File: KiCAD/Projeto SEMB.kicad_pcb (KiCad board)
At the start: 2 copper layers, 153 x 122.5 mm, 90 parts, among them J1 Battery-12V, J2 ST-Link V2, M1 Motor_DC, Q1 IRLML5203, Q2 IRF740, Q3 IRF740, Q4 IRF740, Q5 IRF740, Q6 IRF740, Q7 IRF740, Q8 IRF740, Q9 IRF740, SW1 Reset, SW2 BOOT_0, SW3 SW_SPDT, SW4 User Button, U1 STM32F411CEUx, U10 XL4015, U11 LCD-016N002L, U13 INA333xxDGK, U2 2SMPP-03, U3 TLV2371P, U4 DRV8212P, U5 PCF8574A, U7 TPS7A2433DBVR, Y1 LSE

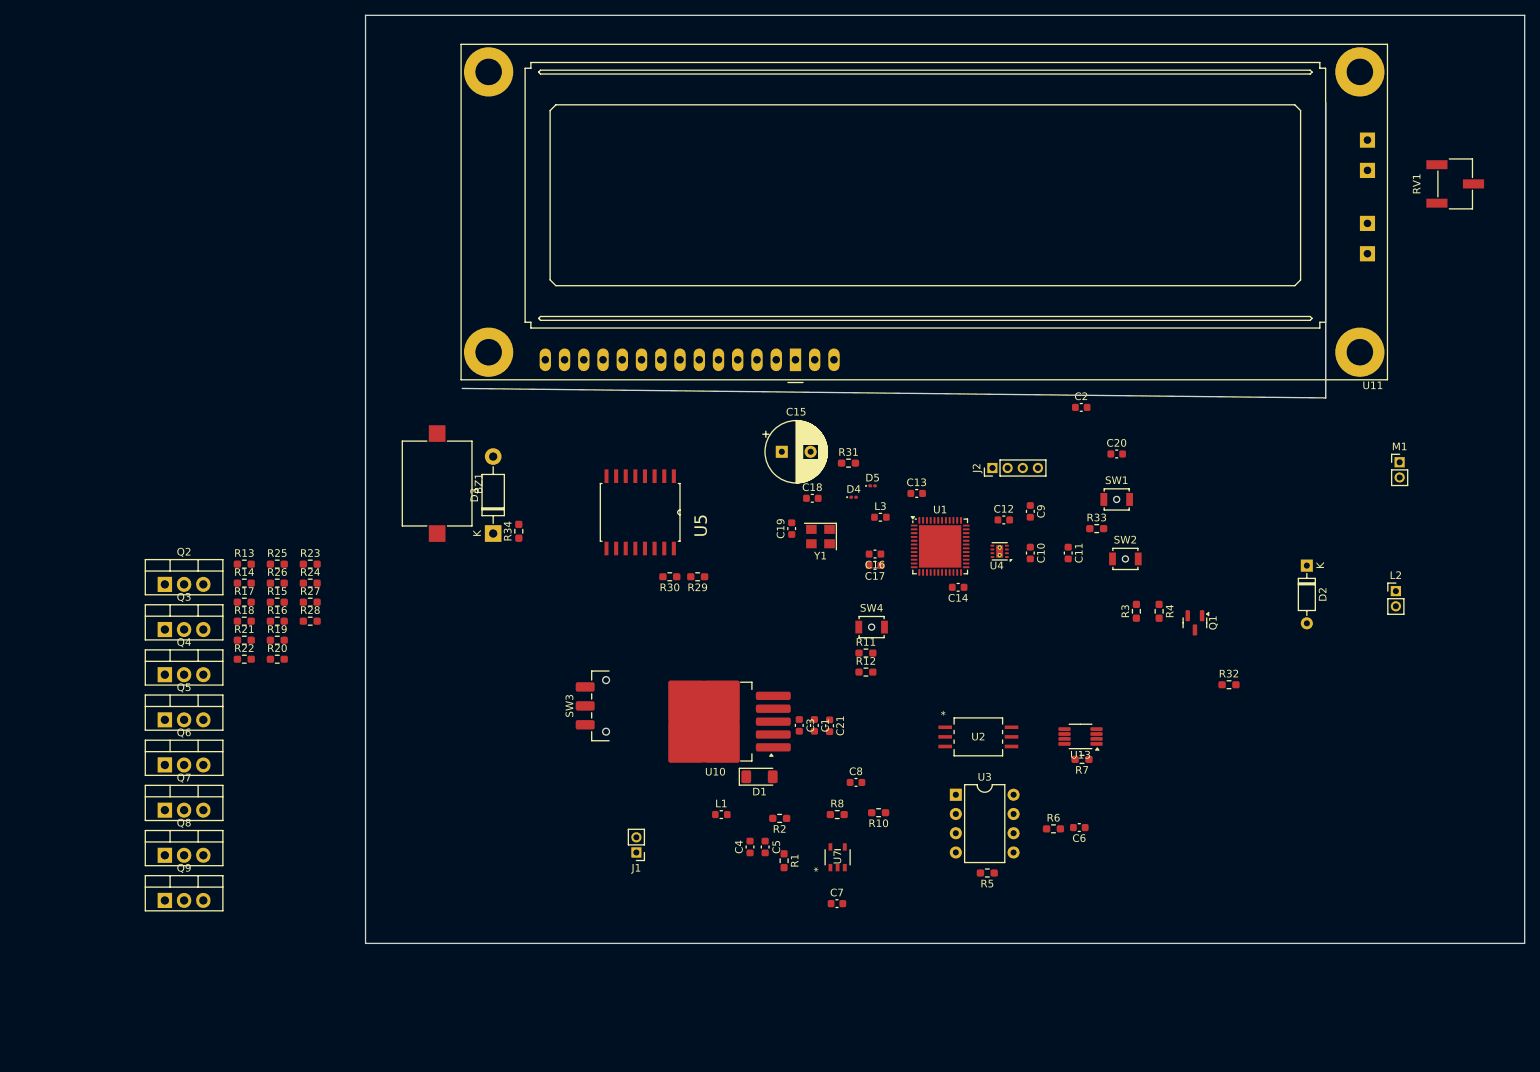
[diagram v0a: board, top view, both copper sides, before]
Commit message: .
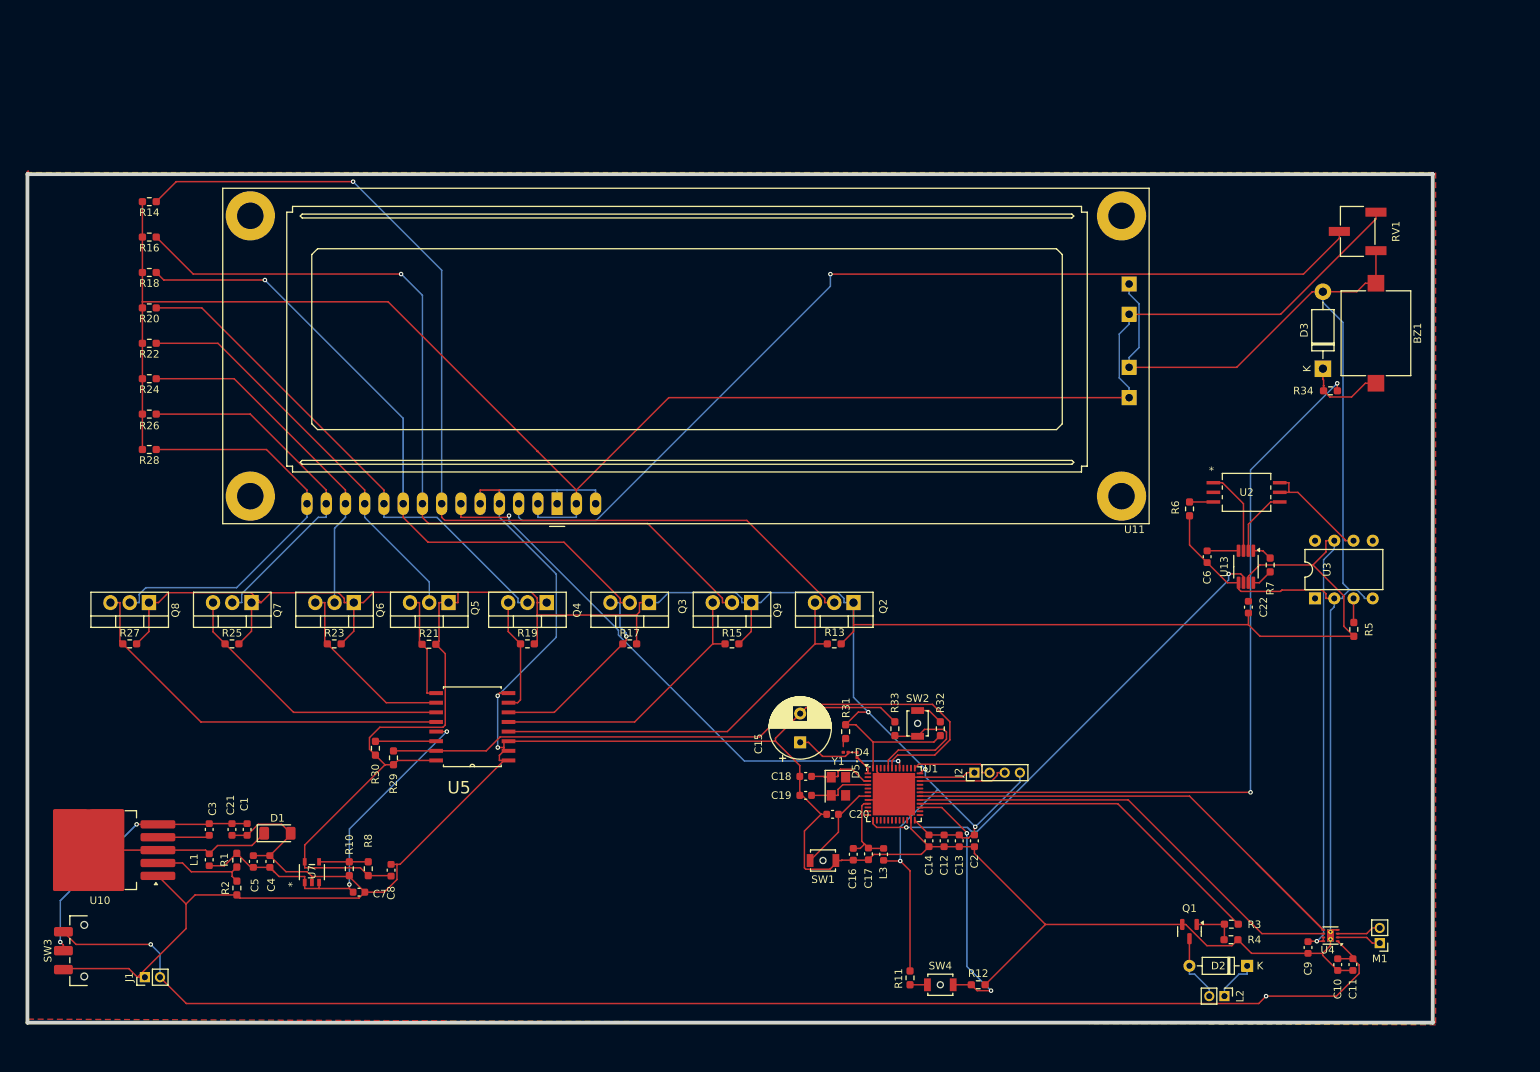
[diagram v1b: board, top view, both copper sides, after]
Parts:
- added C22: 0.1uF, Capacitor_SMD:C_0603_1608Metric, F.Cu at (191.3, 93.4)
- moved BZ1 125.5 mm to (208.1, 57.2)
- moved D3 111.7 mm to (201.1, 61.9)
- moved R34 108.7 mm to (202.1, 64.8), turned to 0 degrees
- moved Q2 90.9 mm to (139.2, 92.8), turned to 180 degrees
- moved Q9 86.8 mm to (125.7, 92.8), turned to 180 degrees
- moved U10 83.0 mm to (39.7, 125.4)
- moved C21 80.1 mm to (57.1, 122.7)
- moved C3 79.1 mm to (54.1, 122.7), turned to -90 degrees
- moved R13 78.6 mm to (136.6, 98.2)
- moved C1 76.1 mm to (59.1, 122.7)
- moved SW3 76.1 mm to (37.6, 138.7)
- moved R1 72.2 mm to (57.8, 126.8)
- moved R2 72.2 mm to (57.8, 130.4), turned to -90 degrees
- moved R10 70.3 mm to (72.6, 127.9), turned to -90 degrees
- moved U7 69.4 mm to (67.7, 128.3)
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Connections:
- C6 pad 1: GND -> Net-(U13-V-)
- U13 pad 4: GND -> Net-(U13-V-)
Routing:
- net GND: track 0.00 -> 556.8 mm, vias 0 -> 2
- net +3.3V: track 0.00 -> 474.3 mm, vias 0 -> 5
- net +5V: track 0.00 -> 291.9 mm, vias 0 -> 2
- net +12V: track 0.00 -> 185.9 mm, vias 0 -> 2
- net DB0: track 0.00 -> 133.1 mm, vias 0 -> 1
- net Net-(U11-VO): track 0.00 -> 127.6 mm, vias 0 -> 1
- net DB1: track 0.00 -> 113.5 mm, vias 0 -> 1
- net PA10: track 0.00 -> 103.4 mm, vias 0 -> 2
- net PB7: track 0.00 -> 89.1 mm
- net DB2: track 0.00 -> 88.5 mm, vias 0 -> 1
- net PB5: track 0.00 -> 74.8 mm, vias 0 -> 2
- net PA9: track 0.00 -> 73.0 mm
- net DB3: track 0.00 -> 67.6 mm
- net PA3: track 0.00 -> 65.3 mm, vias 0 -> 2
- net PA8: track 0.00 -> 60.5 mm
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- added copper zone on F.Cu, net GND
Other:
- board size 153 x 122.5 mm -> 185.5 x 112 mm

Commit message: substitute
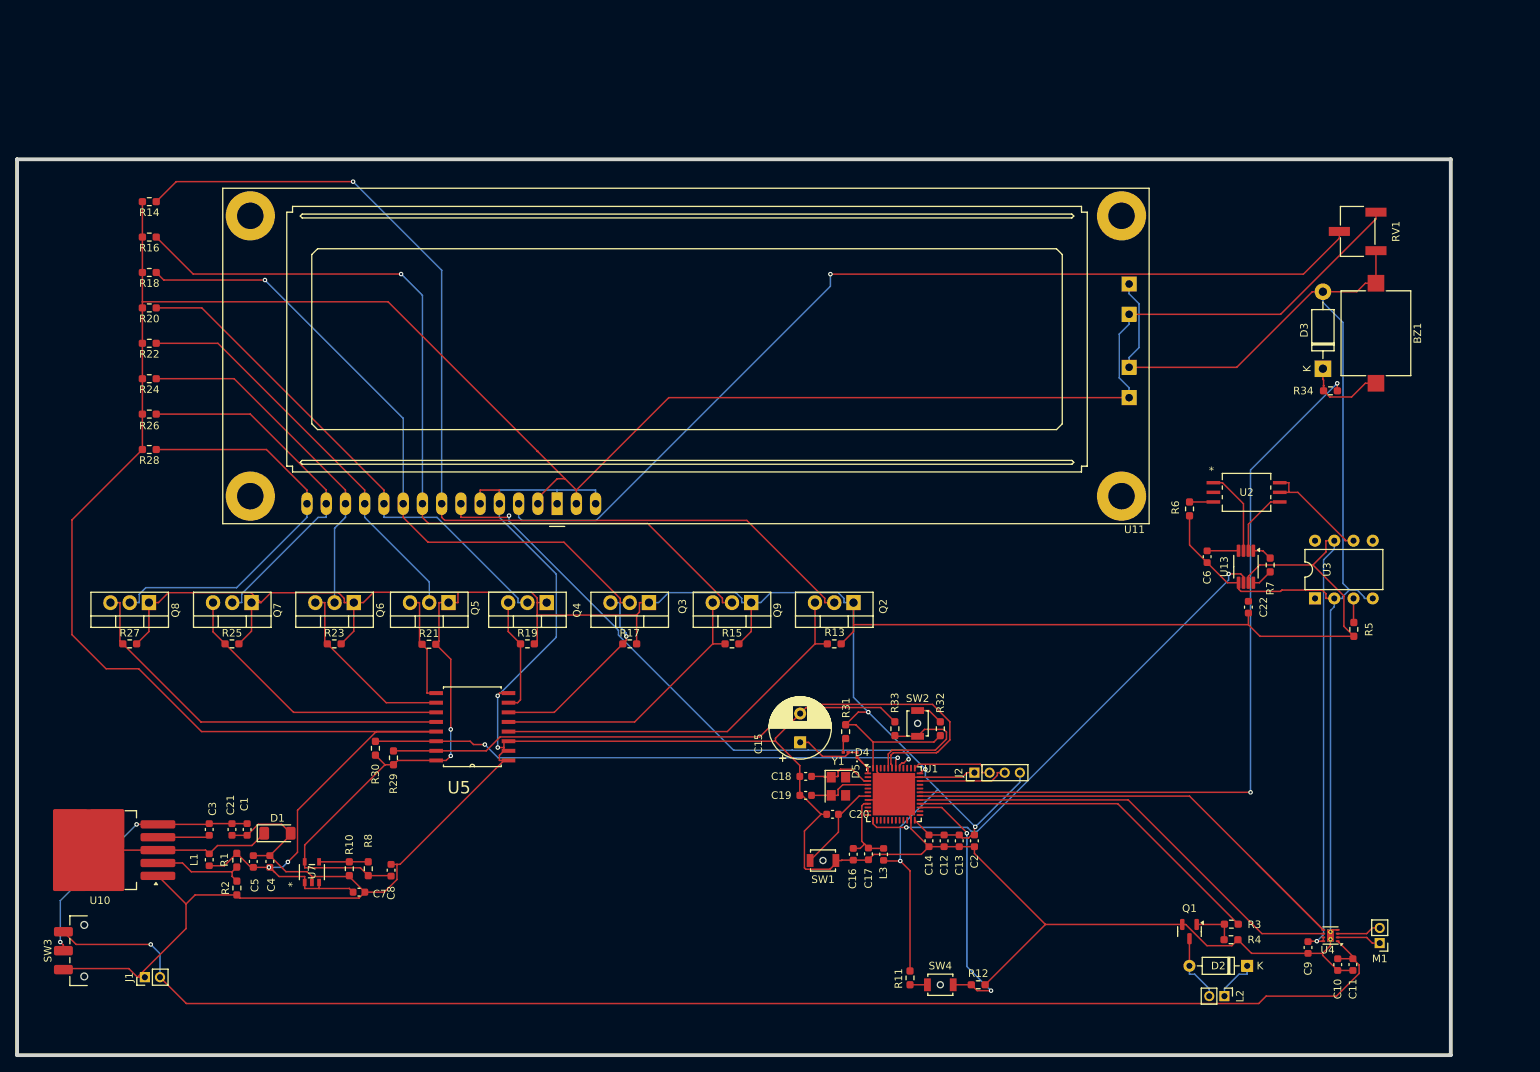
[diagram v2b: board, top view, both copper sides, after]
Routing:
- net +5V: track 291.9 -> 376.0 mm
- net PB6: track 8.02 -> 71.3 mm, vias 0 -> 2
- net +3.3V: track 474.3 -> 467.7 mm, vias 5 -> 7
- net PB5: track 74.8 -> 77.2 mm
- net Net-(D4-A): track 1.52 -> 2.49 mm
- net PB7: track 89.1 -> 89.7 mm
- net +12V: vias 2 -> 1
- removed copper zone on F.Cu, net GND
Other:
- board size 185.5 x 112 mm -> 189.2 x 118.2 mm
